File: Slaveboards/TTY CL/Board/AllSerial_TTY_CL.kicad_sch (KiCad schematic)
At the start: 25 parts, among them Q2 BC857SMD, Q4 BC857SMD, Q5 BC857SMD, T1 BC847, T4 BC847, X1 ALLSERIALSLAVE, X2 AKL18X-08W

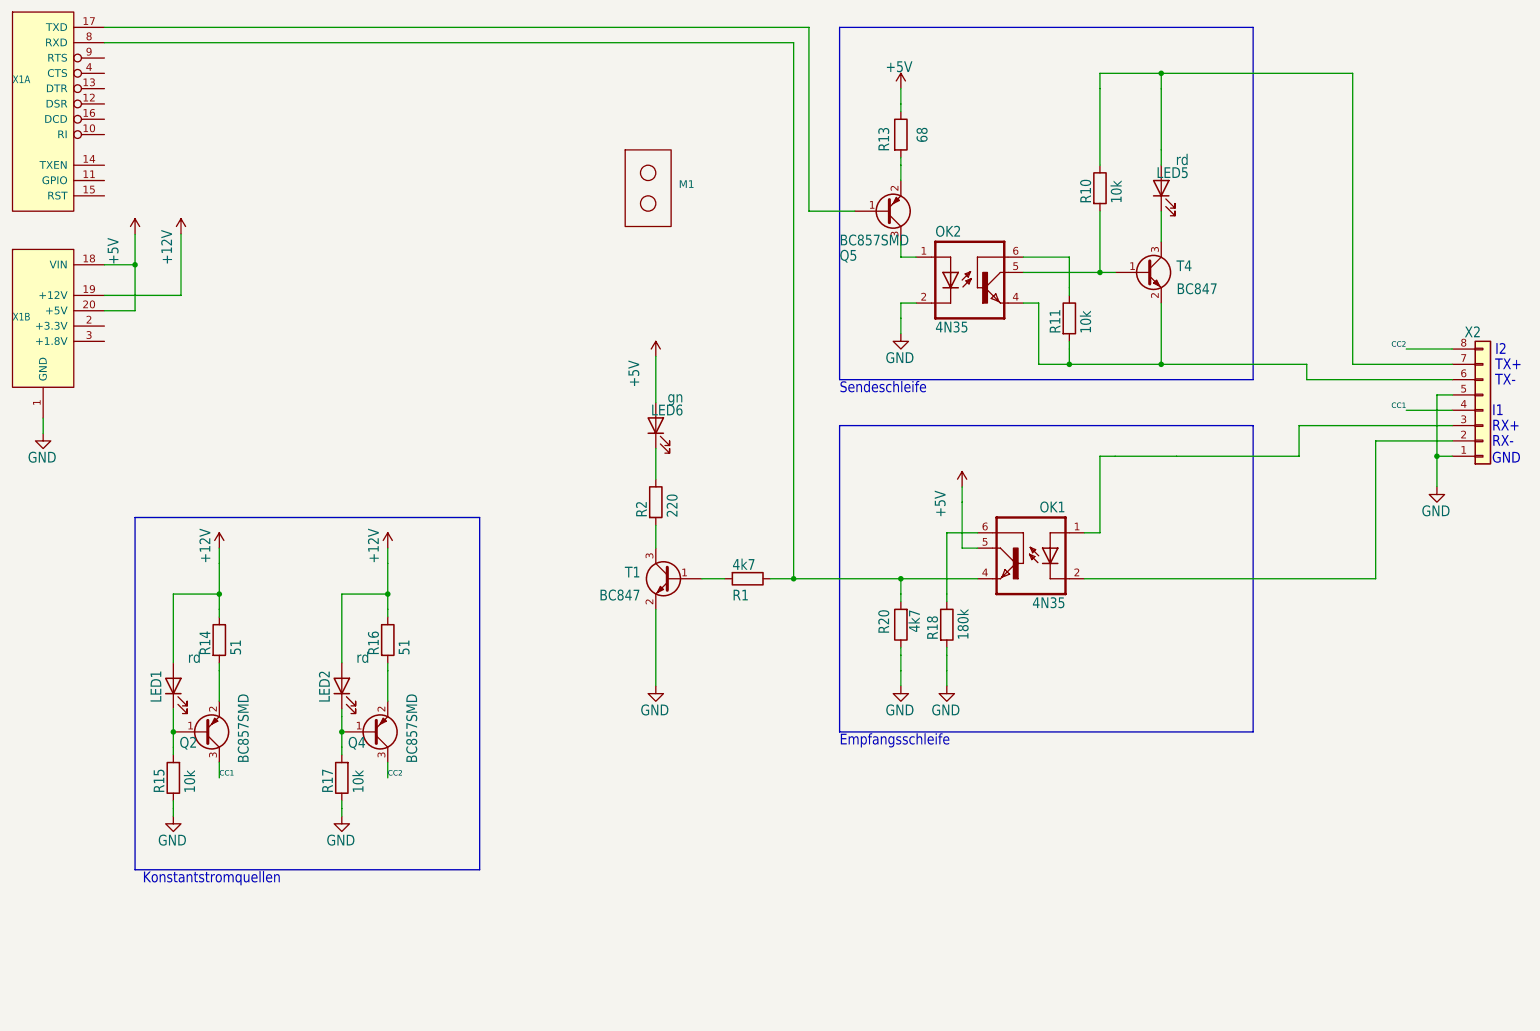
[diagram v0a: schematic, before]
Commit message: Improve libraries
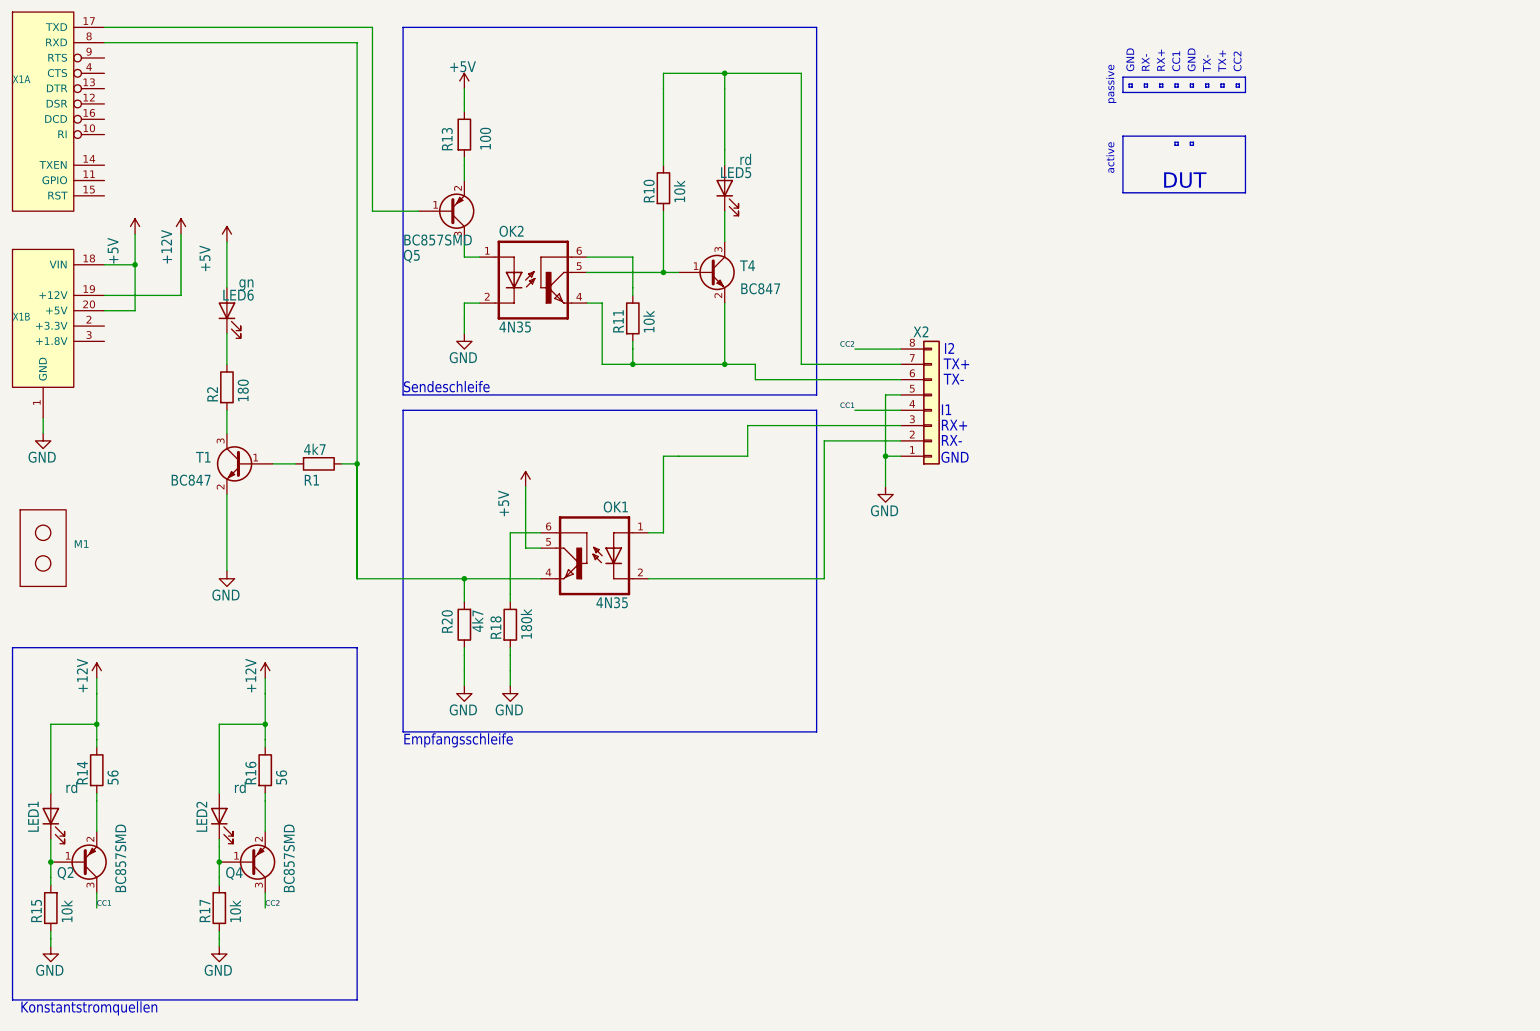
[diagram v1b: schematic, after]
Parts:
- R13: value 68 -> 100
- R14, R16: value 51 -> 56
- R2: value 220 -> 180
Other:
- note added: "CC1"
- note added: "CC2"
- note added: "DUT"
- note added: "active"
- note added: "passive"
- moved on the sheet: LED1, LED2, LED5, LED6, M1, OK1, OK2, Q2, Q4, Q5, R1, R10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
